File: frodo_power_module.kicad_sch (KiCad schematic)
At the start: 61 parts, among them J1 Keystone 1098, J10 SWD Header, J2 Molex MicroFit 2x2, J3 Molex MicroFit 2x2, J4 Molex MicroFit 2x2, J5 Molex MicroFit 2x2, J6 Molex MicroFit 2x2, J7 JST-GH, J8 JST-GH, J9 JST-GH, U1 STM32F042F6Px, U2 L7805, U3 AZ1117I-3.3, U4 BQ25171-Q1, U5 BQ29200, U6 MCP2562-E-SN, Y1 8MHz

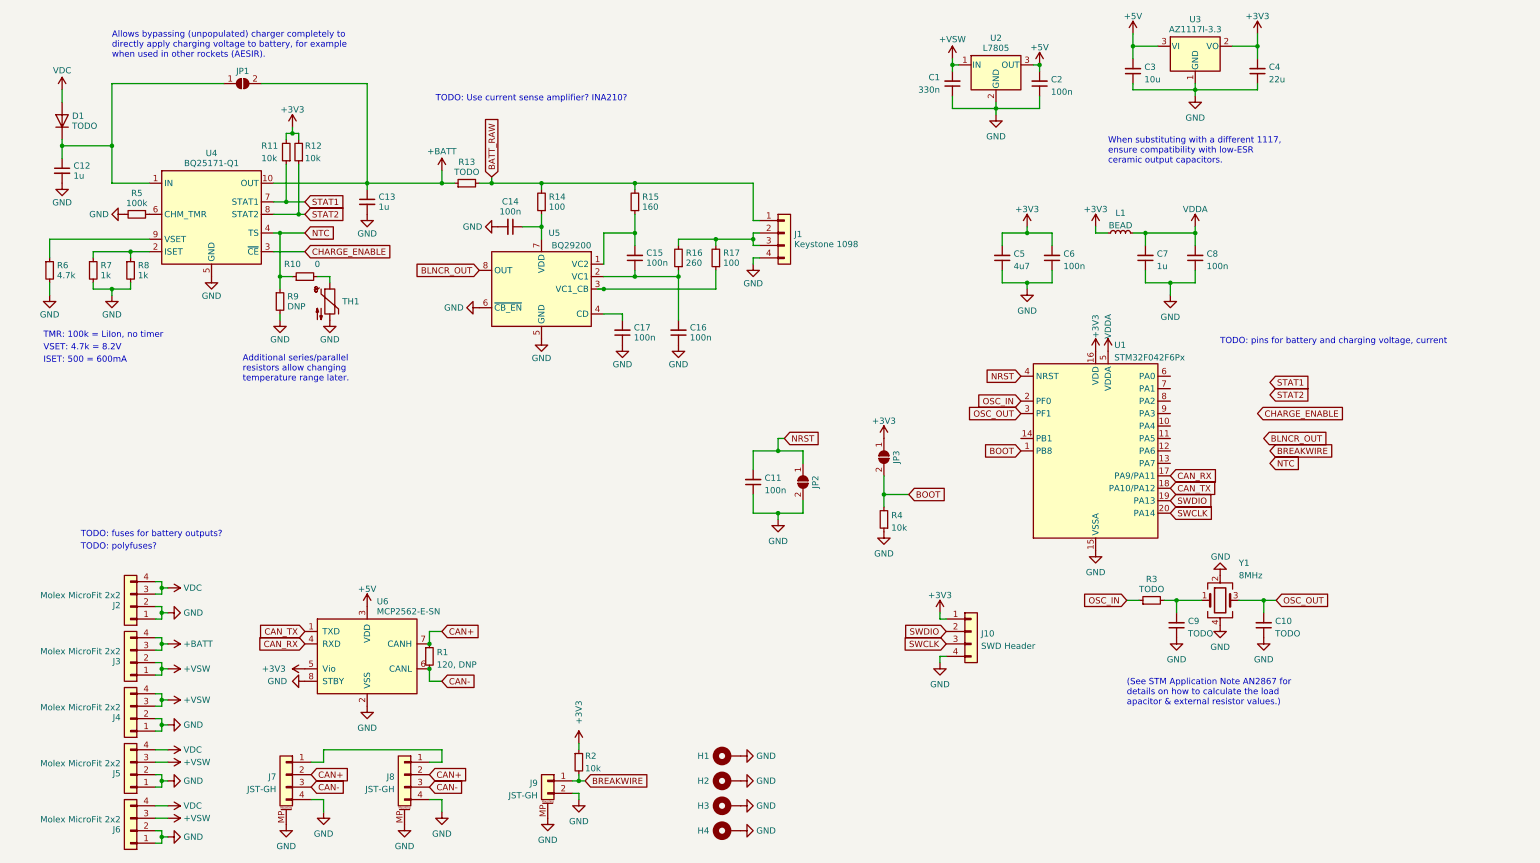
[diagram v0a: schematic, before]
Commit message: Update PCB
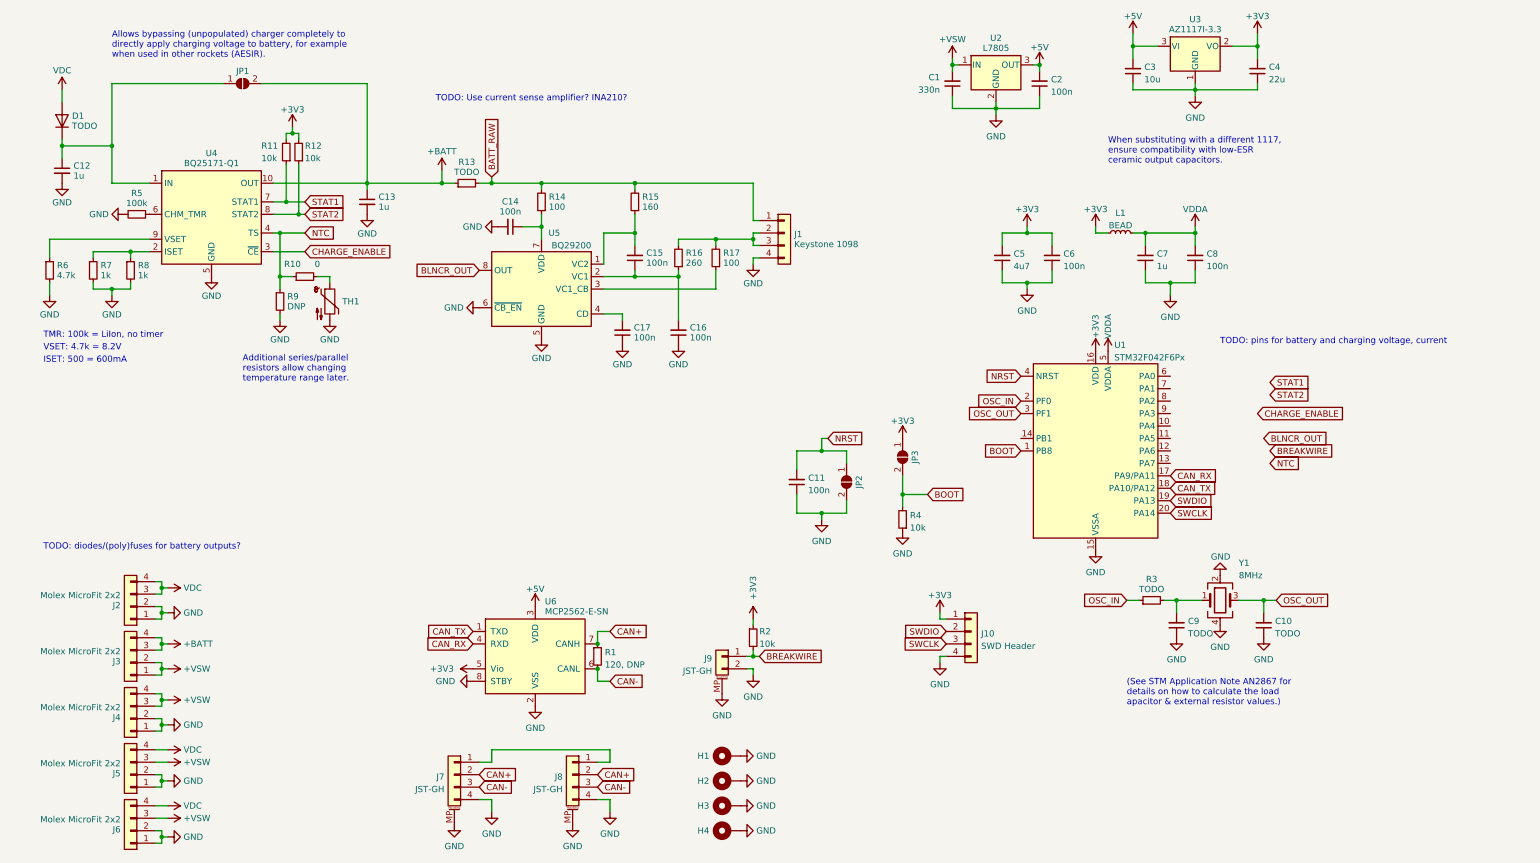
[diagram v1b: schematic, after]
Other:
- note added: "TODO: diodes/(poly)fuses for battery outputs?"
- note removed: "TODO: fuses for battery outputs?"
- note removed: "TODO: polyfuses?"
- moved on the sheet: C11, J7, J8, J9, JP2, JP3, R1, R2, R4, U6
